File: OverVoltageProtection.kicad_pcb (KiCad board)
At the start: 2 copper layers, 36.5 x 28 mm, 0 parts

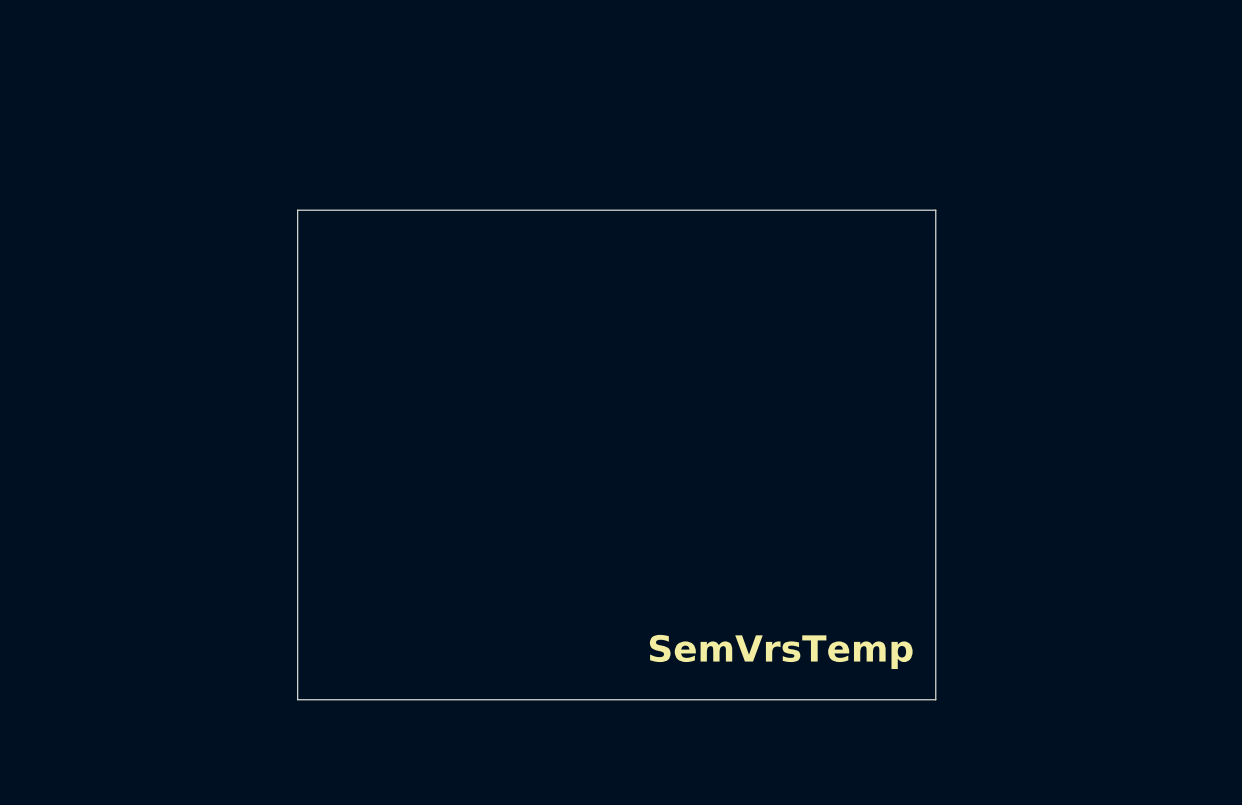
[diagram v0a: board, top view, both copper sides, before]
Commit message: finished layout
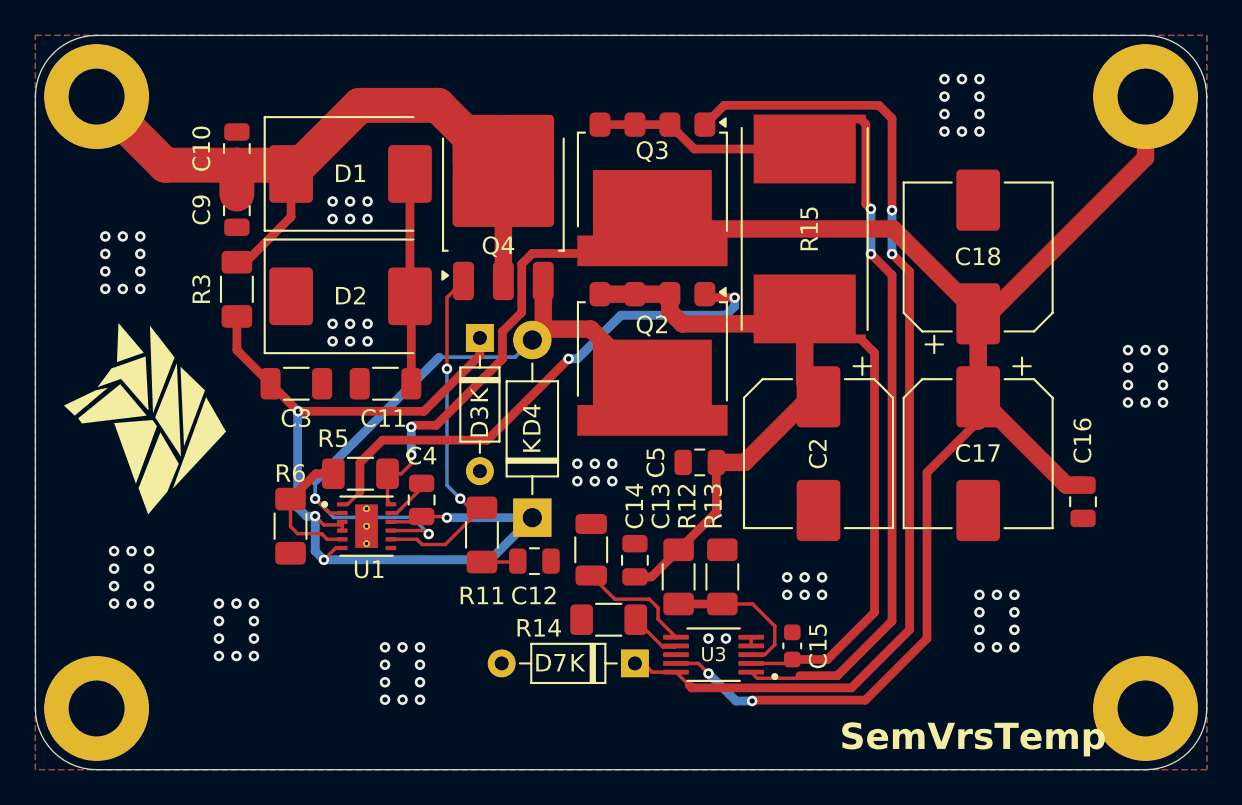
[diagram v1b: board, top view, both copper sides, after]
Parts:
- added C10: 100nF, Capacitor_SMD:C_0805_2012Metric, F.Cu at (54.0, 42.0)
- added C11: 1uF, Capacitor_SMD:C_1206_3216Metric, F.Cu at (62.5, 55.4)
- added C12: 10nF, Capacitor_SMD:C_0805_2012Metric, F.Cu at (71.0, 65.6)
- added C13: 100nF, Capacitor_SMD:C_0805_2012Metric, F.Cu at (76.8, 65.5)
- added C14: 0.56uF, Capacitor_SMD:C_1206_3216Metric, F.Cu at (74.3, 64.9)
- added C15: 1000pF, Capacitor_SMD:C_0603_1608Metric, F.Cu at (85.8, 70.4)
- added C16: 100nF, Capacitor_SMD:C_0805_2012Metric, F.Cu at (102.4, 62.2)
- added C17: 100uF, Capacitor_SMD:CP_Elec_8x10, F.Cu at (96.4, 59.4)
- added C18: 100uF, Capacitor_SMD:CP_Elec_8x10, F.Cu at (96.4, 48.2)
- added C2: 47uF, Capacitor_SMD:CP_Elec_8x10, F.Cu at (87.3, 59.4)
- added C3: 1uF, Capacitor_SMD:C_1206_3216Metric, F.Cu at (57.4, 55.4)
- added C4: 100nF, Capacitor_SMD:C_0805_2012Metric, F.Cu at (64.6, 62.1)
- added C5: 2.2uF, Capacitor_SMD:C_0805_2012Metric, F.Cu at (80.5, 59.9)
- added C9: 100nF, Capacitor_SMD:C_0805_2012Metric, F.Cu at (54.0, 45.5)
- added D1: 5.0SMDJ120A, Diode_SMD:D_SMC, F.Cu at (60.5, 43.4)
- added D2: 5.0SMDJ33CA, Diode_SMD:D_SMC, F.Cu at (60.5, 50.4)
- added D3: 1N6263, Diode_THT:D_DO-35_SOD27_P7.62mm_Horizontal, F.Cu at (67.9, 52.8)
- added D4: 1N4002, Diode_THT:D_DO-41_SOD81_P10.16mm_Horizontal, F.Cu at (70.9, 63.1)
- added D7: 1N6263, Diode_THT:D_DO-35_SOD27_P7.62mm_Horizontal, F.Cu at (76.8, 71.4)
- added H1: MountingHole_M3_3.2mm_Pad, PCM_SL_Mechanical:MountingHole_3.2mm_Pad, F.Cu at (46.0, 74.0)
- added H2: MountingHole_M3_3.2mm_Pad, PCM_SL_Mechanical:MountingHole_3.2mm_Pad, F.Cu at (46.0, 39.0)
- added H3: MountingHole_M3_3.2mm_Pad, PCM_SL_Mechanical:MountingHole_3.2mm_Pad, F.Cu at (106.0, 39.0)
- added H4: MountingHole_M3_3.2mm_Pad, PCM_SL_Mechanical:MountingHole_3.2mm_Pad, F.Cu at (106.0, 74.0)
- added Q2: SQJQ466E, Package_TO_SOT_SMD:LFPAK88, F.Cu at (77.8, 54.1)
- added Q3: SQJQ466E, Package_TO_SOT_SMD:LFPAK88, F.Cu at (77.8, 44.4)
- added Q4: IRFR210PBF, Package_TO_SOT_SMD:TO-252-3_TabPin2, F.Cu at (69.3, 44.5)
- added R11: 100R, Resistor_SMD:R_1206_3216Metric_Pad1.30x1.75mm_HandSolder, F.Cu at (68.0, 64.1)
- added R12: 95.3k, Resistor_SMD:R_1206_3216Metric_Pad1.30x1.75mm_HandSolder, F.Cu at (79.3, 66.5)
- added R13: 13.7k, Resistor_SMD:R_1206_3216Metric_Pad1.30x1.75mm_HandSolder, F.Cu at (81.8, 66.5)
- added R14: 54.9k, Resistor_SMD:R_1206_3216Metric_Pad1.30x1.75mm_HandSolder, F.Cu at (75.3, 68.9)
- added R15: 0.004R, Resistor_SMD:R_Shunt_Vishay_WSR2_WSR3_KelvinConnection, F.Cu at (86.8, 46.6)
- added R3: 10k, Resistor_SMD:R_1206_3216Metric_Pad1.30x1.75mm_HandSolder, F.Cu at (54.0, 50.0)
- added R5: 100k, Resistor_SMD:R_1206_3216Metric_Pad1.30x1.75mm_HandSolder, F.Cu at (61.1, 60.6)
- added R6: 3.48K, Resistor_SMD:R_1206_3216Metric_Pad1.30x1.75mm_HandSolder, F.Cu at (57.1, 63.6)
- added U1: LM74800QDRRRQ1, LM74800QDRRRQ1:IC_LM74800QDRRRQ1, F.Cu at (61.4, 63.6)
- added U3: LM5069MM-2_NOPB, LM5069MM-2_NOPB:SOP50P490X110-10N, F.Cu at (81.3, 70.9)
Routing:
- net V_FILTERED: track 0.00 -> 103.8 mm, vias 0 -> 4
- net Net-(D7-K): track 0.00 -> 58.3 mm, vias 0 -> 2
- net /V_INTER: track 0.00 -> 56.3 mm
- net /VS: track 0.00 -> 53.4 mm, vias 0 -> 4
- net /SENSE: track 0.00 -> 51.2 mm, vias 0 -> 2
- net VBat: track 0.00 -> 41.6 mm
- net /OUT: track 0.00 -> 36.4 mm, vias 0 -> 2
- net /DGATE: track 0.00 -> 30.1 mm, vias 0 -> 2
- net /HGATE: track 0.00 -> 20.1 mm, vias 0 -> 2
- net Net-(C11-+): track 0.00 -> 11.9 mm
- net /UVLO: track 0.00 -> 8.67 mm
- net Net-(R5--): track 0.00 -> 7.88 mm
- net Net-(C14-+): track 0.00 -> 6.69 mm
- net Net-(R14-+): track 0.00 -> 2.97 mm
- net Net-(C4--): track 0.00 -> 2.35 mm
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- added copper zone on B.Cu, net GND
- added copper zone on F.Cu, net GND
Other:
- board size 36.5 x 28 mm -> 67 x 42 mm
